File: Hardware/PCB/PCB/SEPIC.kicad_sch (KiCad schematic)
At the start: 16 parts, among them Q1 IRF7807, U1 LM3478MA

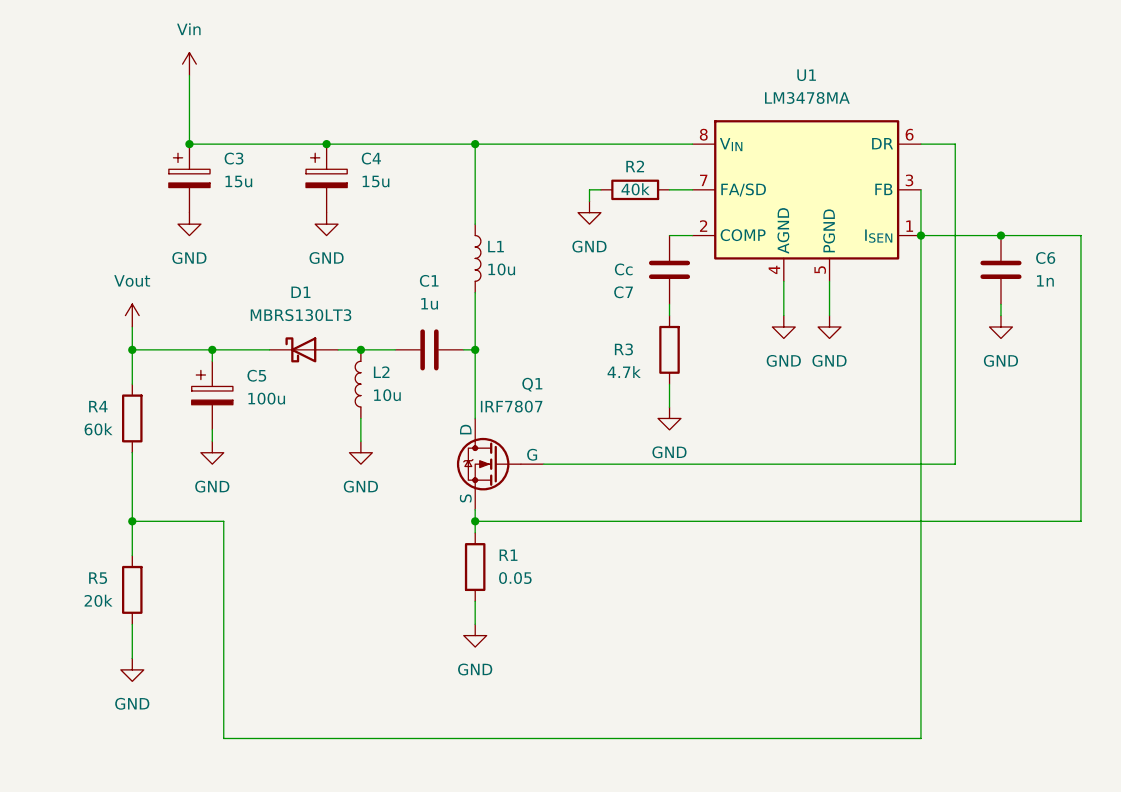
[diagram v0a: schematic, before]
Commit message: Basic schematic
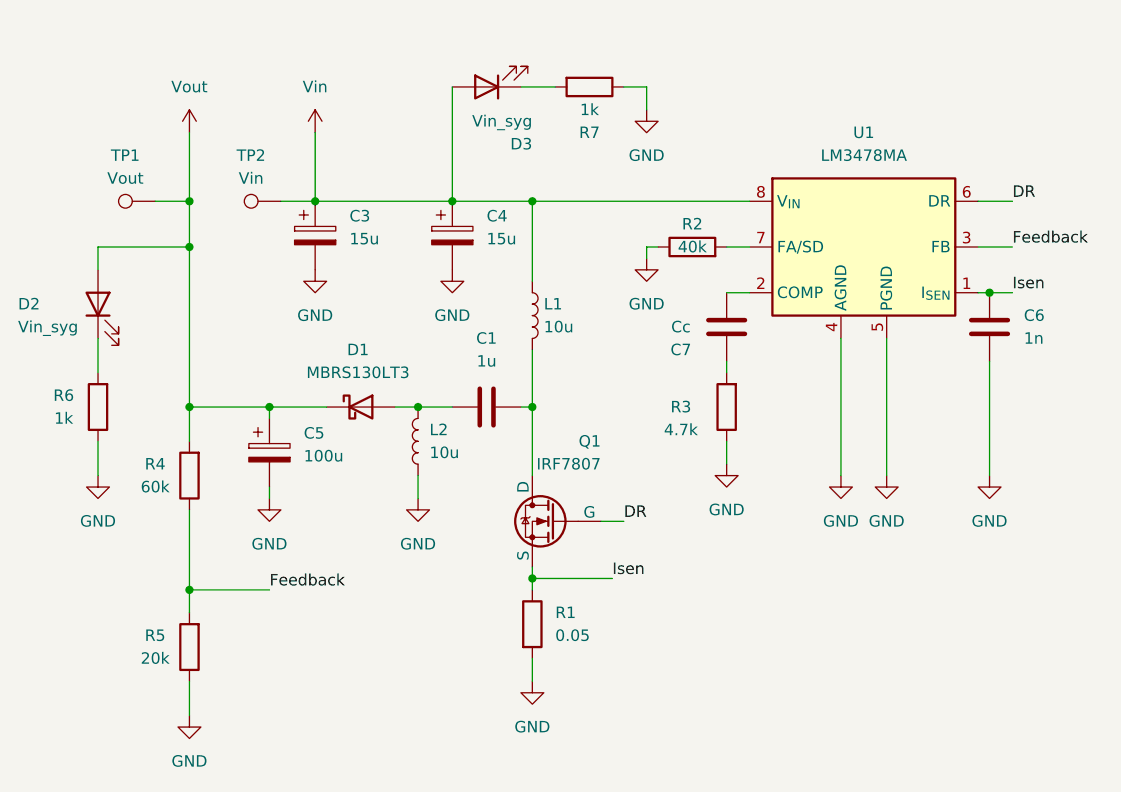
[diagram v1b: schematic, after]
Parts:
- added D2, D3: Vin_syg, symbol Device:LED
- added R6, R7: 1k, symbol Device:R
- added TP1: Vout, Connector_Pin:Pin_D1.0mm_L10.0mm, symbol Connector:TestPoint
- added TP2: Vin, Connector_Pin:Pin_D1.0mm_L10.0mm, symbol Connector:TestPoint
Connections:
- net GND: now also R6.1, R7.1
- net Vin: now also D3.2 (A), TP2.1
- net Vout: now also D2.2 (A), TP1.1
- net Isen: now reaches C6.2, Q1.3 (S), R1.1, U1.1 (I_{SEN})
- net Isen: no longer R4.1, R5.2, U1.3 (FB)
- net DR: now reaches Q1.2 (G), U1.6 (DR)
- new net: D2.1 (K), R6.2
- new net: D3.1 (K), R7.2
- new net Feedback: R4.1, R5.2, U1.3 (FB)
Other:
- moved on the sheet: C1, C3, C4, C5, C6, C7, D1, L1, L2, Q1, R1, R2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
